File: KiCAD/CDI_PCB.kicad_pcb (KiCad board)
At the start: 2 copper layers, 86.9 x 77.7 mm, 45 parts, among them P1 Blue, P10 Green w/ White, P11 Pink, P2 Black w/ White, P3 Yellow, P4 Green Coil, P5 Green Harness, P6 White, P7 Orange, P8 Brown, P9 Light Blue

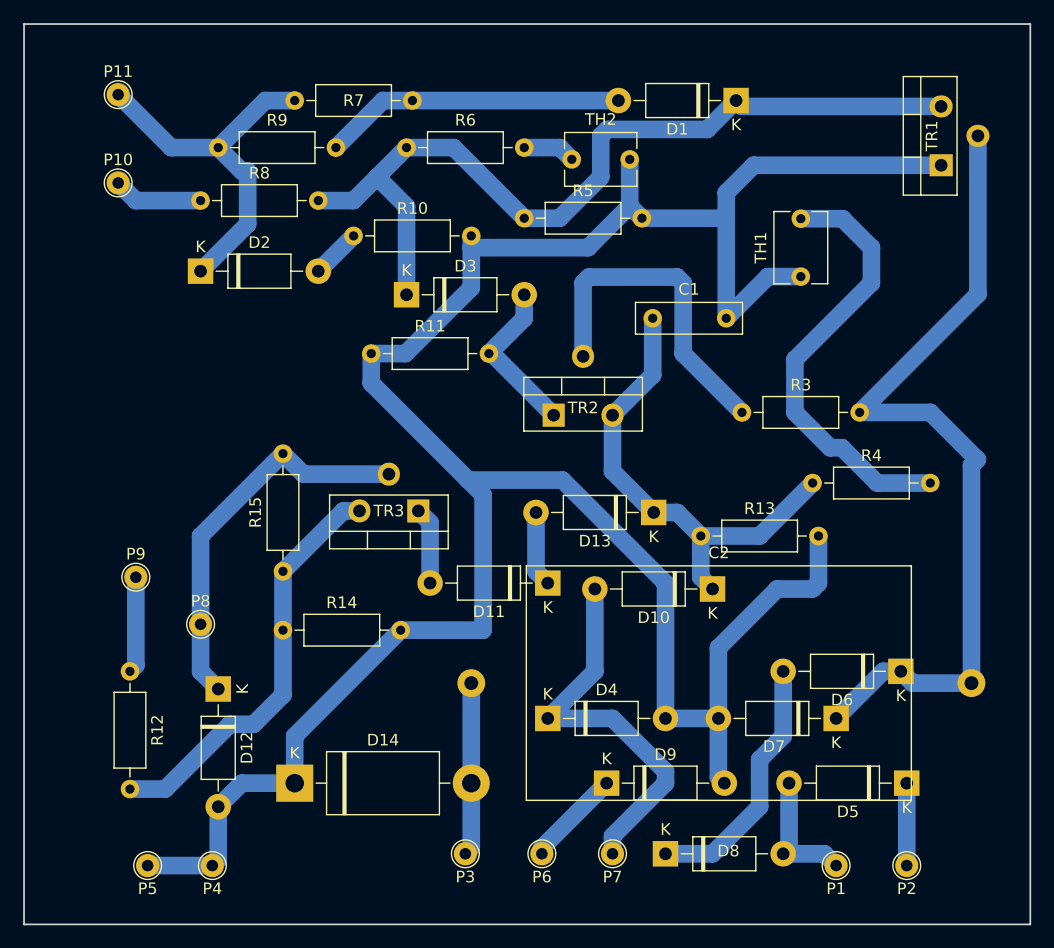
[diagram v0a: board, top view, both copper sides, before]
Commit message: Shrink it down another 0.5in
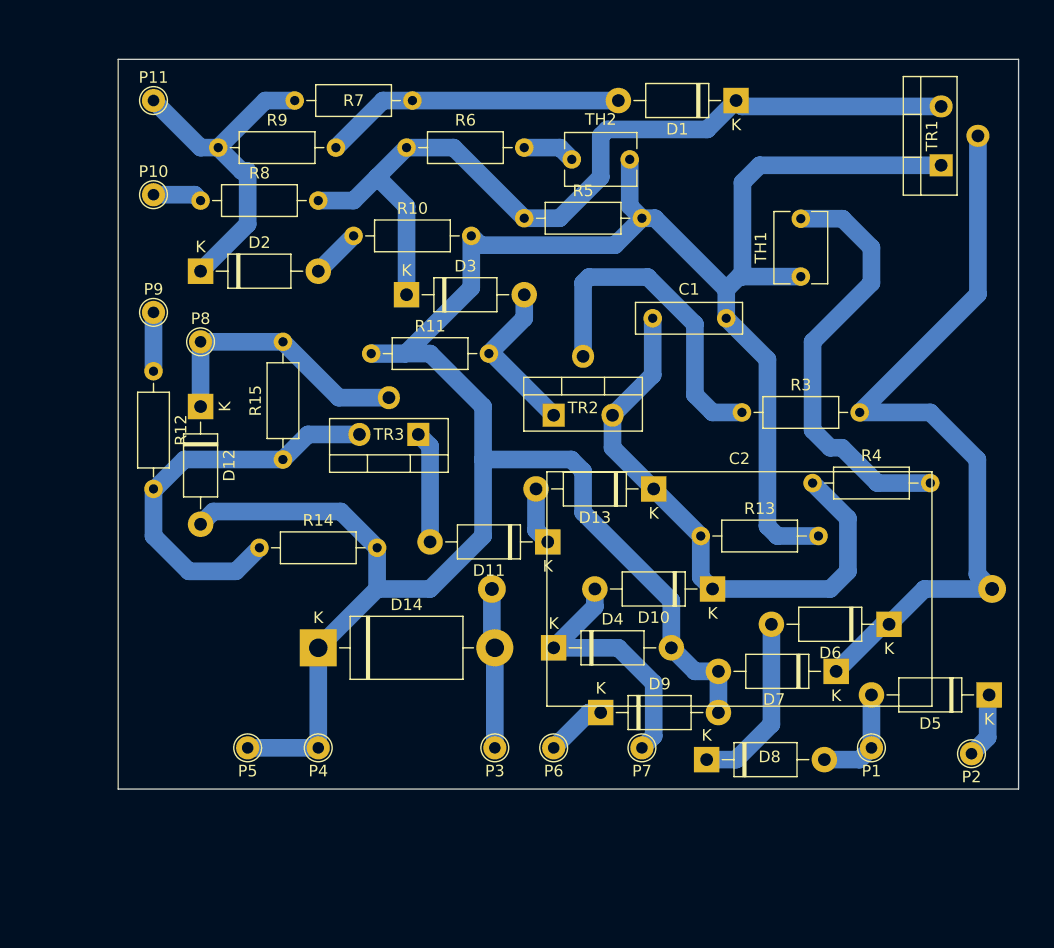
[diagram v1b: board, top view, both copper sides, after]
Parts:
- moved R12 26.0 mm to (111.8, 71.1)
- moved D12 24.4 mm to (115.8, 74.2)
- moved P8 24.4 mm to (115.8, 68.6)
- moved P9 22.9 mm to (111.8, 66.0)
- moved P4 13.7 mm to (126.0, 103.6)
- moved P5 13.3 mm to (119.9, 103.6)
- moved D14 11.9 mm to (126.0, 95.0)
- moved P2 11.2 mm to (182.4, 104.1)
- moved P1 10.6 mm to (173.7, 103.6)
- moved D5 10.4 mm to (183.9, 99.1)
- moved R15 9.65 mm to (122.9, 78.7)
- moved P7 9.49 mm to (153.9, 103.6)
- moved P3 9.49 mm to (141.2, 103.6)
- moved P6 9.20 mm to (146.3, 103.6)
- moved D8 8.87 mm to (159.5, 104.6)
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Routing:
- net Net-(D10-Pad2): track 33.9 -> 22.5 mm
- net Net-(D12-Pad1): track 33.8 -> 23.8 mm
- net Net-(C1-Pad1): track 41.1 -> 49.6 mm
- net Net-(D6-Pad2): track 22.3 -> 15.5 mm
- net Net-(C2-Pad2): track 73.3 -> 68.1 mm
- net Net-(P10-Pad1): track 7.74 -> 4.27 mm
- net Net-(P9-Pad1): track 8.34 -> 5.08 mm
- net Net-(D2-Pad1): track 32.5 -> 29.3 mm
- net Net-(D9-Pad1): track 8.41 -> 5.33 mm
- net Net-(D11-Pad2): track 6.65 -> 9.70 mm
- net Net-(C1-Pad2): track 216.0 -> 218.4 mm
- net Net-(D5-Pad2): track 11.3 -> 9.06 mm
- net Net-(D11-Pad1): track 6.52 -> 4.99 mm
- net Net-(D5-Pad1): track 7.11 -> 5.66 mm
- net Net-(R4-Pad2): track 38.3 -> 37.0 mm
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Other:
- board size 86.9 x 77.7 mm -> 77.7 x 63 mm
